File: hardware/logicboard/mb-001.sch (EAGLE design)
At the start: 31 parts, among them IC1 74ALS05N, IC2 LTC485N, IC3 LTC485N, J0 DC5V, J1 DIN5, J2 DIN5, J3 DIN5, X1 NELTRON-7810-XPXC, X2 NELTRON-7810-XPXC

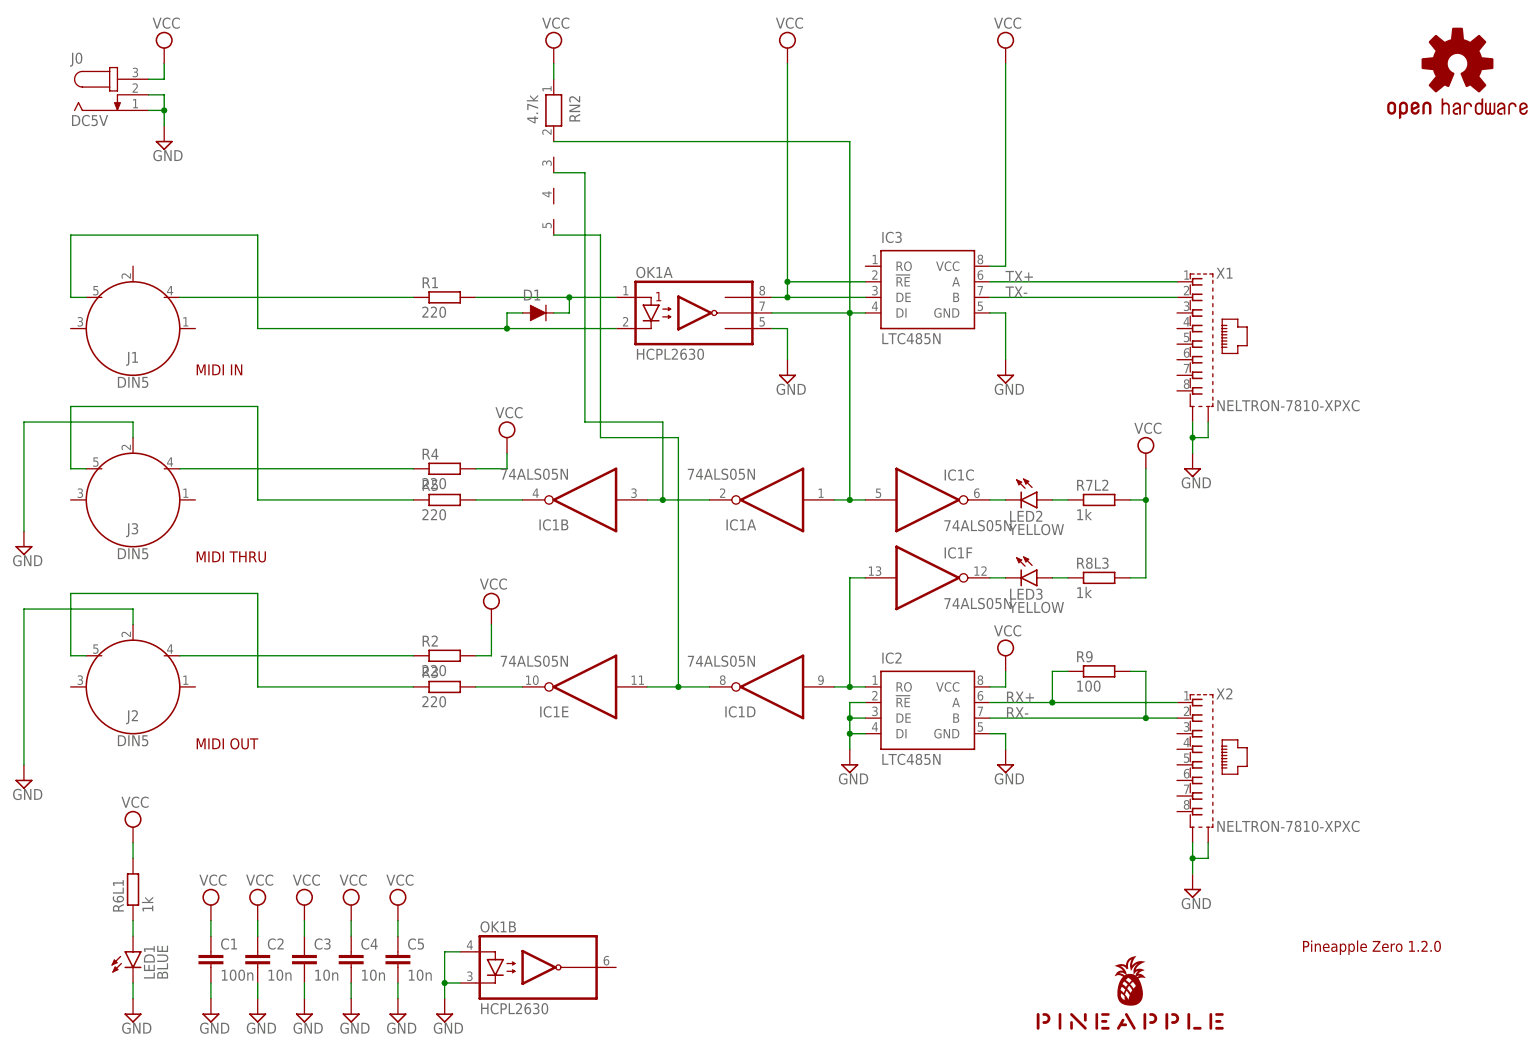
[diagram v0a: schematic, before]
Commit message: Initial design.
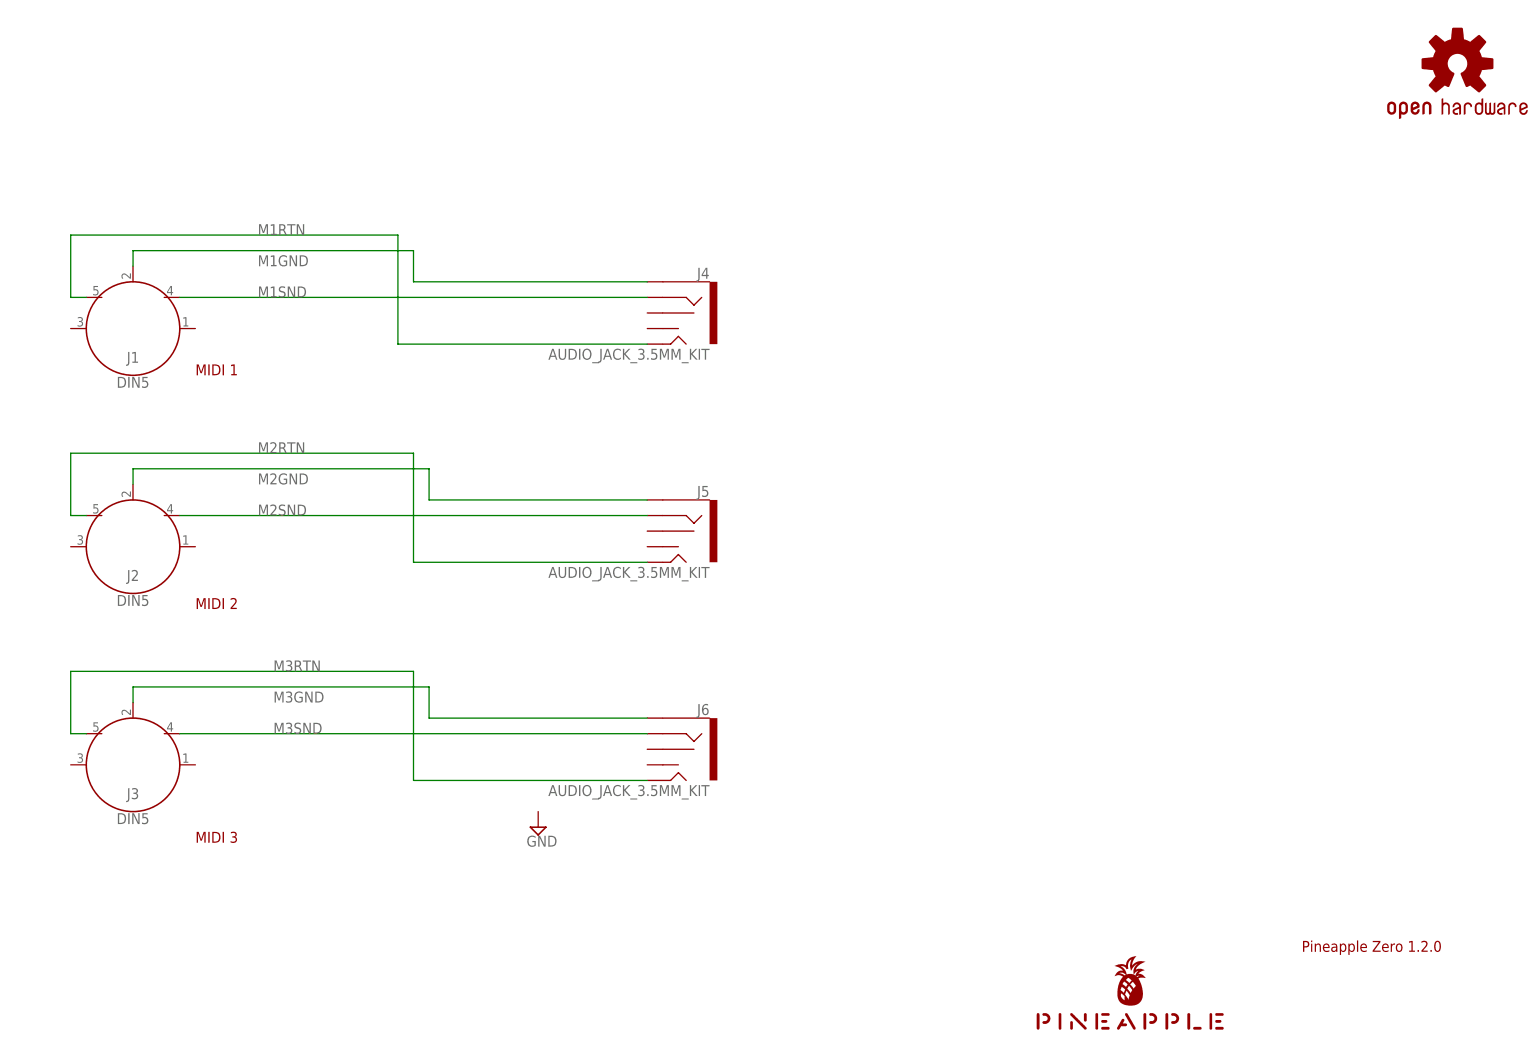
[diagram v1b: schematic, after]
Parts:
- removed C1: 100n, rcl:C-EU025-024X044
- removed C2, C3, C4, C5: 10n, rcl:C-EU025-024X044
- removed D1: DIODE-1N4148, SparkFun-DiscreteSemi:DIODE-1N4148
- removed IC1: 74ALS05N, 74xx-us:74ALS05N
- removed IC2, IC3: LTC485N, linear-technology:LTC485N
- removed J0: DC5V, con-jack:JACK-PLUG0
- removed LED1: BLUE, led:LED3MM
- removed LED2, LED3: YELLOW, led:LED3MM
- removed OK1: HCPL2630, optocoupler:HCPL2630
- removed R1, R2, R3, R4, R5: 220, rcl:R-EU_0204/5
- removed R6L1, R7L2, R8L3: 1k, rcl:R-EU_0204/5
- removed R9: 100, rcl:R-EU_0204/5
- removed RN2: 4.7k, resistor-net:RN04
- removed X1, X2: NELTRON-7810-XPXC, con-rj45:NELTRON-7810-XPXC
- added J4, J5, J6: AUDIO_JACK_3.5MM_KIT, SparkFun-Connectors:AUDIO_JACK_3.5MM_KIT
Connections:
- removed net GND: C1.2, C2.2, C3.2, C4.2, C5.2, IC2.!RE, IC2.DE, IC2.DI, IC2.GND, IC3.GND, J0.1, J0.2, J2.2, J3.2, LED1.C, OK1A.GND, OK1B.A2, OK1B.C2, X1.S1, X1.S2, X2.S1, X2.S2
- removed net MIDIIN: D1.C, OK1A.A1, R1.2
- removed net MIDIOUT: IC1E.O, R3.2
- removed net MIDITHRU: IC1B.O, R5.2
- removed net MIRTN: D1.A, J1.5, OK1A.C1
- removed net MISND: J1.4, R1.1
- removed net MORTN: J2.5, R3.1
- removed net MOSND: J2.4, R2.1
- removed net MTRTN: J3.5, R5.1
- removed net MTSND: J3.4, R4.1
- removed net N$1: IC1C.O, LED2.C
- removed net N$2: LED3.A, R8L3.1
- removed net N$3: IC1F.O, LED3.C
- removed net N$4: LED1.A, R6L1.1
- removed net N$5: LED2.A, R7L2.1
- removed net NMIDIOUT: IC1D.O, IC1E.I, RN2.5
- removed net NMIDITHRU: IC1A.O, IC1B.I, RN2.3
- removed net RX: IC1D.I, IC1F.I, IC2.RO
- removed net RX+: IC2.A, R9.1, X2.1
- removed net RX-: IC2.B, R9.2, X2.2
- removed net TX: IC1A.I, IC1C.I, IC3.DI, OK1A.VO1, RN2.2
- removed net TX+: IC3.A, X1.1
- removed net TX-: IC3.B, X1.2
- removed net VCC: C1.1, C2.1, C3.1, C4.1, C5.1, IC2.VCC, IC3.!RE, IC3.DE, IC3.VCC, J0.3, OK1A.VCC, R2.2, R4.2, R6L1.2, R7L2.2, R8L3.2, RN2.1
- new net M1GND: J1.2, J4.SLEEVE
- new net M1RTN: J1.5, J4.TIP
- new net M1SND: J1.4, J4.RING
- new net M2GND: J2.2, J5.SLEEVE
- new net M2RTN: J2.5, J5.TIP
- new net M2SND: J2.4, J5.RING
- new net M3GND: J3.2, J6.SLEEVE
- new net M3RTN: J3.5, J6.TIP
- new net M3SND: J3.4, J6.RING
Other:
- note added: "MIDI 1"
- note added: "MIDI 2"
- note added: "MIDI 3"
- note removed: "MIDI IN"
- note removed: "MIDI OUT"
- note removed: "MIDI THRU"
- moved on the sheet: J2, J3
